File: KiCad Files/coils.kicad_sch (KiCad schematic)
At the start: 13 parts, among them Q1 AO3400A, Q2 AO3400A, Q3 AO3400A, Q4 AO3400A, Q5 AO3401A, Q6 AO3401A, Q7 AO3401A, Q8 AO3401A, U2 74HC595

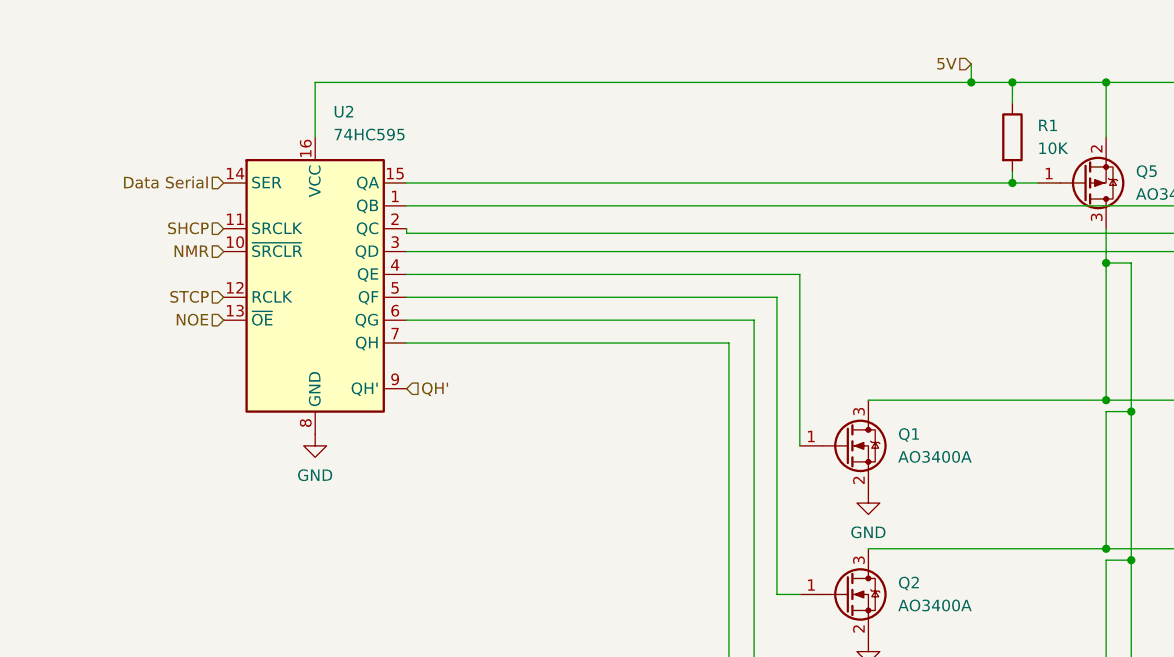
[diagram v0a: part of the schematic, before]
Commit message: Big saucy business
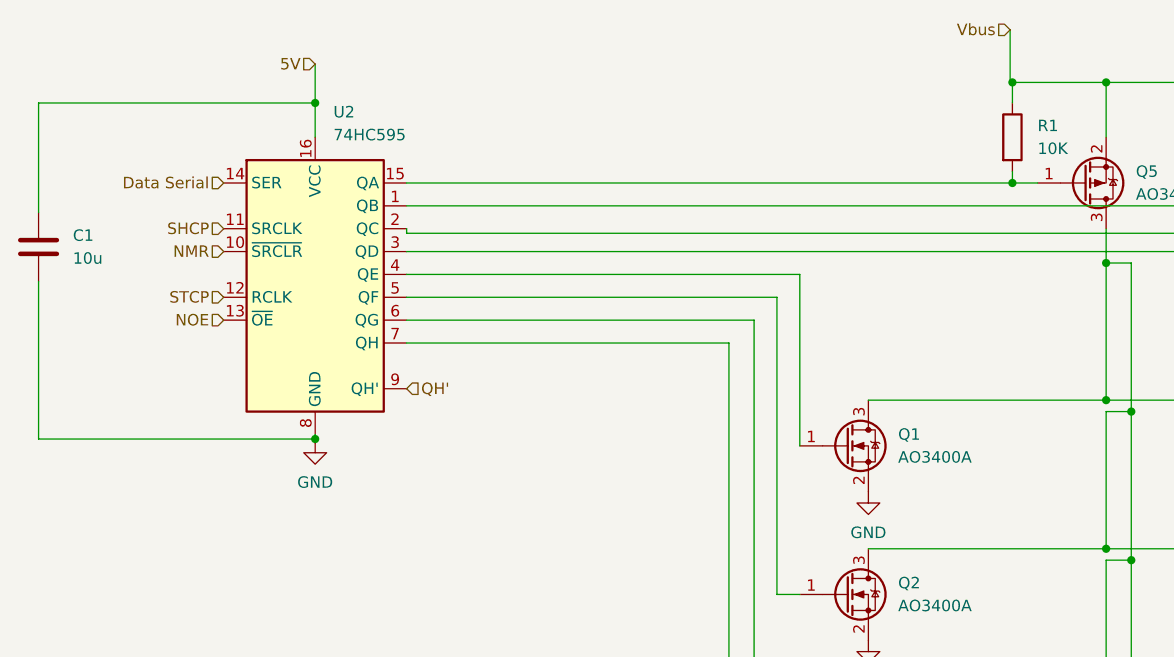
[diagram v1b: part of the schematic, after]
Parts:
- added C1: 10u, Capacitor_SMD:C_0805_2012Metric, symbol Device:C
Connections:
- net 5V: now also C1.1; no longer Q5.2 (S), Q6.2 (S), Q7.2 (S), Q8.2 (S), R1.1, R2.1, R3.1, R4.1
- net GND: now also C1.2
- new net Vbus: Q5.2 (S), Q6.2 (S), Q7.2 (S), Q8.2 (S), R1.1, R2.1, R3.1, R4.1
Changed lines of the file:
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@@
   (junction (at 191.516 87.884) (diameter 0) (color 0 0 0 0)
   )
+  (junction (at 188.722 119.888) (diameter 0) (color 0 0 0 0)
+  )
+  (junction (at 188.722 54.864) (diameter 0) (color 0 0 0 0)
+  )
+  (junction (at 201.676 46.228) (diameter 0) (color 0 0 0 0)
+  )
+  (junction (at 188.722 70.358) (diameter 0) (color 0 0 0 0)
+  )
+  (junction (at 149.86 88.138) (diameter 0) (color 0 0 0 0)
+  )
+  (junction (at 167.386 55.118) (diameter 0) (color 0 0 0 0)
+  )
+  (junction (at 59.182 74.676) (diameter 0) (color 0 0 0 0)
+  )
+  (junction (at 181.102 46.228) (diameter 0) (color 0 0 0 0)
+  )
+  (junction (at 170.18 71.628) (diameter 0) (color 0 0 0 0)
+  )
+  (junction (at 167.386 35.052) (diameter 0) (color 0 0 0 0)
+  )
   (junction (at 136.652 35.052) (diameter 0) (color 0 0 0 0)
   )
-  (junction (at 188.722 119.888) (diameter 0) (color 0 0 0 0)
-  )
-  (junction (at 188.722 54.864) (diameter 0) (color 0 0 0 0)
-  )
-  (junction (at 201.676 46.228) (diameter 0) (color 0 0 0 0)
-  )
-  (junction (at 188.722 70.358) (diameter 0) (color 0 0 0 0)
-  )
-  (junction (at 149.86 88.138) (diameter 0) (color 0 0 0 0)
-  )
-  (junction (at 132.08 35.052) (diameter 0) (color 0 0 0 0)
-  )
-  (junction (at 167.386 55.118) (diameter 0) (color 0 0 0 0)
-  )
-  (junction (at 181.102 46.228) (diameter 0) (color 0 0 0 0)
-  )
-  (junction (at 170.18 71.628) (diameter 0) (color 0 0 0 0)
-  )
-  (junction (at 167.386 35.052) (diameter 0) (color 0 0 0 0)
-  )
   (junction (at 209.296 54.864) (diameter 0) (color 0 0 0 0)
   )
@@
   (junction (at 147.066 103.378) (diameter 0) (color 0 0 0 0)
   )
+  (junction (at 59.182 37.338) (diameter 0) (color 0 0 0 0)
+  )
   (junction (at 178.308 35.052) (diameter 0) (color 0 0 0 0)
   )
@@
     (stroke (width 0) (type default) (color 0 0 0 0))
   )
+  (wire (pts (xy 28.448 49.53) (xy 28.448 37.338))
+    (stroke (width 0) (type default) (color 0 0 0 0))
+  )
   (wire (pts (xy 198.882 44.958) (xy 198.882 46.228))
     (stroke (width 0) (type default) (color 0 0 0 0))
@@
     (stroke (width 0) (type default) (color 0 0 0 0))
   )
-  (wire (pts (xy 59.182 35.052) (xy 59.182 41.148))
+  (wire (pts (xy 59.182 33.02) (xy 59.182 37.338))
     (stroke (width 0) (type default) (color 0 0 0 0))
   )
@@
     (stroke (width 0) (type default) (color 0 0 0 0))
   )
+  (wire (pts (xy 136.398 35.052) (xy 136.652 35.052))
+    (stroke (width 0) (type default) (color 0 0 0 0))
+  )
   (wire (pts (xy 136.652 46.228) (xy 139.446 46.228))
     (stroke (width 0) (type default) (color 0 0 0 0))
@@
     (stroke (width 0) (type default) (color 0 0 0 0))
   )
+  (wire (pts (xy 136.398 29.21) (xy 136.398 35.052))
+    (stroke (width 0) (type default) (color 0 0 0 0))
+  )
   (wire (pts (xy 149.86 104.648) (xy 149.86 88.138))
     (stroke (width 0) (type default) (color 0 0 0 0))
@@
     (stroke (width 0) (type default) (color 0 0 0 0))
   )
-  (wire (pts (xy 132.08 35.052) (xy 136.652 35.052))
-    (stroke (width 0) (type default) (color 0 0 0 0))
-  )
   (wire (pts (xy 212.09 71.374) (xy 209.296 71.374))
     (stroke (width 0) (type default) (color 0 0 0 0))
@@
     (stroke (width 0) (type default) (color 0 0 0 0))
   )
+  (wire (pts (xy 59.182 37.338) (xy 59.182 41.148))
+    (stroke (width 0) (type default) (color 0 0 0 0))
+  )
   (wire (pts (xy 191.516 104.394) (xy 191.516 87.884))
     (stroke (width 0) (type default) (color 0 0 0 0))
@@
     (stroke (width 0) (type default) (color 0 0 0 0))
   )
+  (wire (pts (xy 59.182 74.676) (xy 59.182 74.93))
+    (stroke (width 0) (type default) (color 0 0 0 0))
+  )
   (wire (pts (xy 113.03 108.458) (xy 107.95 108.458))
     (stroke (width 0) (type default) (color 0 0 0 0))
@@
     (stroke (width 0) (type default) (color 0 0 0 0))
   )
+  (wire (pts (xy 28.448 37.338) (xy 59.182 37.338))
+    (stroke (width 0) (type default) (color 0 0 0 0))
+  )
   (wire (pts (xy 170.18 88.138) (xy 170.18 71.628))
     (stroke (width 0) (type default) (color 0 0 0 0))
@@
     (stroke (width 0) (type default) (color 0 0 0 0))
   )
+  (wire (pts (xy 59.182 74.168) (xy 59.182 74.676))
+    (stroke (width 0) (type default) (color 0 0 0 0))
+  )
   (wire (pts (xy 107.95 61.468) (xy 69.342 61.468))
     (stroke (width 0) (type default) (color 0 0 0 0))
@@
     (stroke (width 0) (type default) (color 0 0 0 0))
   )
-  (wire (pts (xy 59.182 35.052) (xy 132.08 35.052))
-    (stroke (width 0) (type default) (color 0 0 0 0))
-  )
   (wire (pts (xy 212.09 71.374) (xy 212.09 54.864))
     (stroke (width 0) (type default) (color 0 0 0 0))
@@
     (stroke (width 0) (type default) (color 0 0 0 0))
   )
+  (wire (pts (xy 28.448 57.15) (xy 28.448 74.676))
+    (stroke (width 0) (type default) (color 0 0 0 0))
+  )
   (wire (pts (xy 209.296 51.308) (xy 209.296 54.864))
     (stroke (width 0) (type default) (color 0 0 0 0))
@@
     (stroke (width 0) (type default) (color 0 0 0 0))
   )
-  (wire (pts (xy 132.08 33.02) (xy 132.08 35.052))
+  (wire (pts (xy 28.448 74.676) (xy 59.182 74.676))
     (stroke (width 0) (type default) (color 0 0 0 0))
   )
@@
     (effects (font (size 1.27 1.27)) (justify left))
   )
-  (hierarchical_label "5V" (shape input) (at 132.08 33.02 180)
+  (hierarchical_label "5V" (shape input) (at 59.182 33.02 180)
     (effects (font (size 1.27 1.27)) (justify right))
   )
@@
     (effects (font (size 1.27 1.27)) (justify right))
   )
+  (hierarchical_label "Vbus" (shape input) (at 136.398 29.21 180)
+    (effects (font (size 1.27 1.27)) (justify right))
+  )
   (symbol (lib_id "Device:R") (at 136.652 41.148 0) (unit 1)
     (in_bom yes) (on_board yes) (fields_autoplaced)
@@
   (symbol (lib_id "power:GND") (at 120.65 97.028 0) (unit 1)
     (in_bom yes) (on_board yes) (fields_autoplaced)
-    (property "Reference" "#PWR04" (id 0) (at 120.65 103.378 0)
+    (property "Reference" "#PWR07" (id 0) (at 120.65 103.378 0)
       (effects (font (size 1.27 1.27)) hide)
     )
@@
   (symbol (lib_id "power:GND") (at 120.65 130.048 0) (unit 1)
     (in_bom yes) (on_board yes) (fields_autoplaced)
-    (property "Reference" "#PWR06" (id 0) (at 120.65 136.398 0)
+    (property "Reference" "#PWR09" (id 0) (at 120.65 136.398 0)
       (effects (font (size 1.27 1.27)) hide)
     )
@@
   (symbol (lib_id "power:GND") (at 120.65 80.518 0) (unit 1)
     (in_bom yes) (on_board yes) (fields_autoplaced)
-    (property "Reference" "#PWR03" (id 0) (at 120.65 86.868 0)
+    (property "Reference" "#PWR06" (id 0) (at 120.65 86.868 0)
       (effects (font (size 1.27 1.27)) hide)
     )
@@
     (pin "3")
   )
-  (symbol (lib_id "power:GND") (at 59.182 74.168 0) (unit 1)
-    (in_bom yes) (on_board yes) (fields_autoplaced)
-    (property "Reference" "#PWR02" (id 0) (at 59.182 80.518 0)
-      (effects (font (size 1.27 1.27)) hide)
-    )
-    (property "Value" "GND" (id 1) (at 59.182 78.74 0))
-    (property "Footprint" "" (id 2) (at 59.182 74.168 0)
-      (effects (font (size 1.27 1.27)) hide)
-    )
-    (property "Datasheet" "" (id 3) (at 59.182 74.168 0)
+  (symbol (lib_id "Device:C") (at 28.448 53.34 0) (unit 1)
+    (in_bom yes) (on_board yes) (fields_autoplaced)
+    (property "Reference" "C1" (id 0) (at 32.258 52.0699 0)
+      (effects (font (size 1.27 1.27)) (justify left))
+    )
+    (property "Value" "10u" (id 1) (at 32.258 54.6099 0)
+      (effects (font (size 1.27 1.27)) (justify left))
+    )
+    (property "Footprint" "Capacitor_SMD:C_0805_2012Metric" (id 2) (at 29.4132 57.15 0)
+      (effects (font (size 1.27 1.27)) hide)
+    )
+    (property "Datasheet" "https://datasheet.lcsc.com/lcsc/1811121310_Samsung-Electro-Mechanics-CL21A106KAYNNNE_C15850.pdf" (id 3) (at 28.448 53.34 0)
+      (effects (font (size 1.27 1.27)) hide)
+    )
+    (property "JLC Part Number" "C15850" (id 4) (at 28.448 53.34 0)
+      (effects (font (size 1.27 1.27)) hide)
+    )
+    (pin "1")
+    (pin "2")
+  )
+  (symbol (lib_id "power:GND") (at 59.182 74.93 0) (unit 1)
+    (in_bom yes) (on_board yes) (fields_autoplaced)
+    (property "Reference" "#PWR05" (id 0) (at 59.182 81.28 0)
+      (effects (font (size 1.27 1.27)) hide)
+    )
+    (property "Value" "GND" (id 1) (at 59.182 79.502 0))
+    (property "Footprint" "" (id 2) (at 59.182 74.93 0)
+      (effects (font (size 1.27 1.27)) hide)
+    )
+    (property "Datasheet" "" (id 3) (at 59.182 74.93 0)
       (effects (font (size 1.27 1.27)) hide)
     )
@@
   (symbol (lib_id "power:GND") (at 120.65 113.538 0) (unit 1)
     (in_bom yes) (on_board yes) (fields_autoplaced)
-    (property "Reference" "#PWR05" (id 0) (at 120.65 119.888 0)
-      (effects (font (size 1.27 1.27)) hide)
-    )
+    (property "Reference" "#PWR08" (id 0) (at 120.65 119.888 0)
+      (effects (font (size 1.27 1.27)) hide)
+    )
